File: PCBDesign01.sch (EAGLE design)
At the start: 94 parts, among them IC1 TESEO-LIV3R, J1 5051102491ACTUAL, U1 TPS71913-28DRVR, U2 FXOS8700CQR1, U3 CD40109BPWR, U4 MCP23017T-E/SO

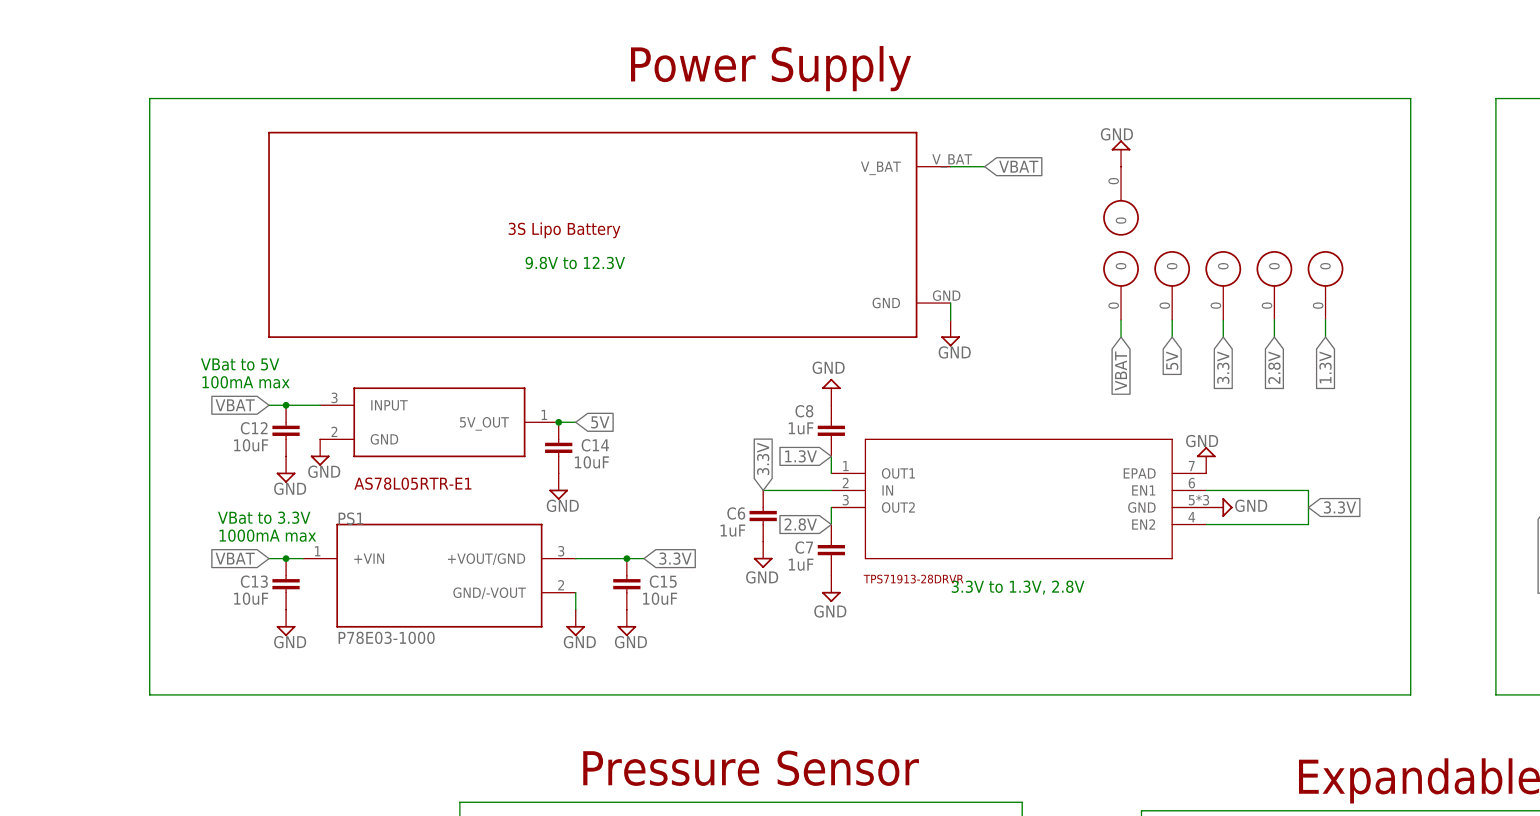
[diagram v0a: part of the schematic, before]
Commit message: final?
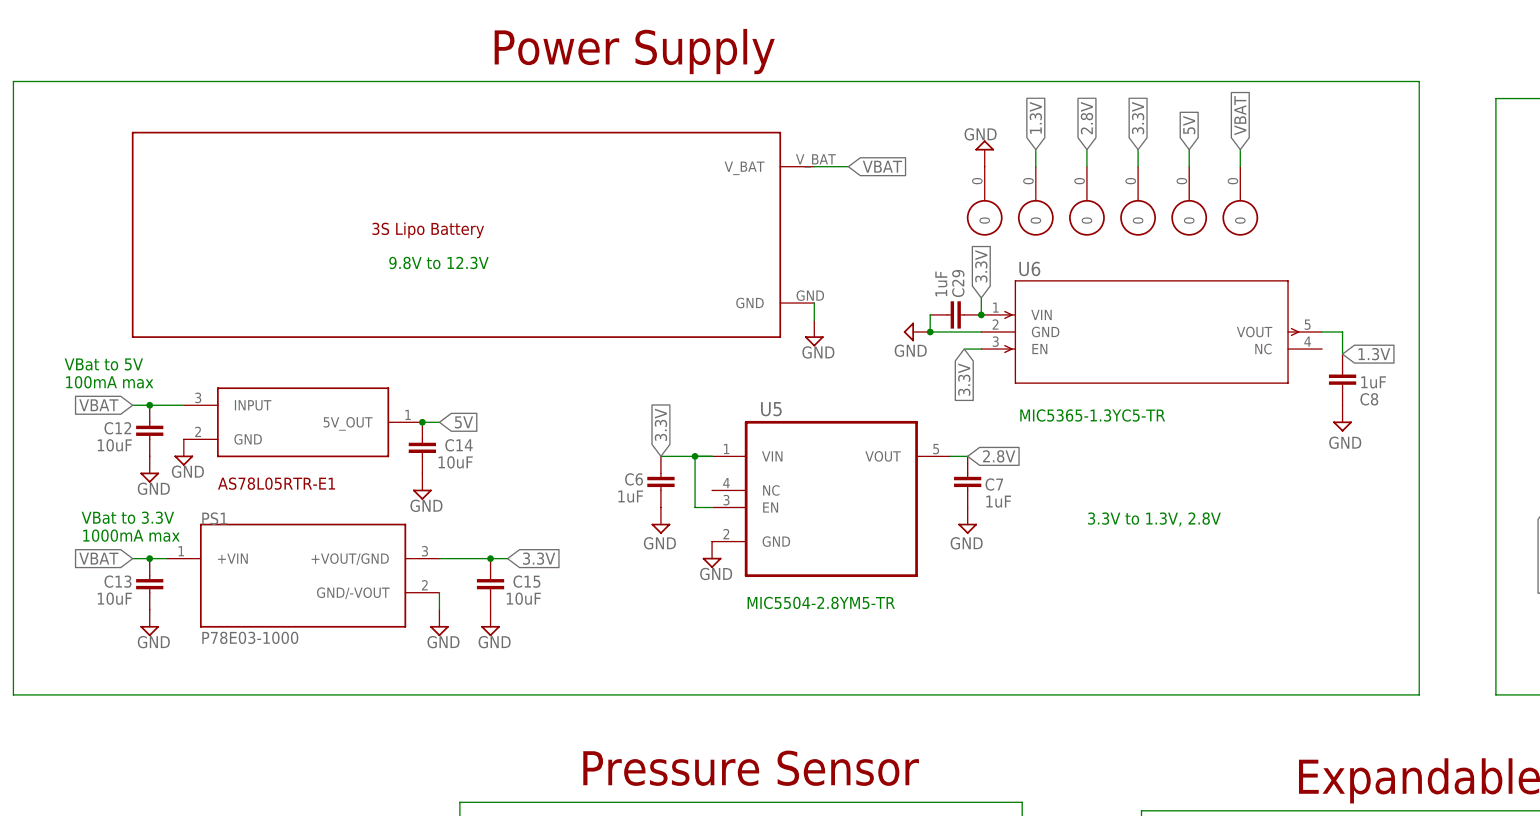
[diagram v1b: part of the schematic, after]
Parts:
- removed U1: TPS71913-28DRVR, TPS71913-28DRVR:TPS71913-28DRVR
- added C29: 1uF, Capacitor:C_CHIP-0805(2012-METRIC)
- added U5: MIC5504-2.8YM5-TR, MIC5504_2.8YM5:MIC5504-2.8YM5-TR
- added U6: MIC5365-1.3YC5-TRSC-70_C5_MCH-M, MIC5365_1.3YC5:MIC5365-1.3YC5-TRSC-70_C5_MCH-M
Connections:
- net 1.3V: now also U6.VOUT; no longer U1.OUT1
- net 2.8V: now also U5.VOUT; no longer U1.OUT2
- net 3.3V: now also C29.1, U5.EN, U5.VIN, U6.EN, U6.VIN; no longer U1.EN1, U1.EN2, U1.IN
- net GND: now also C29.2, U5.GND, U6.GND; no longer U1.EPAD, U1.GND
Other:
- note added: "MIC5365-1.3YC5-TR"
- note added: "MIC5504-2.8YM5-TR"
- moved on the sheet: C12, C13, C14, C15, C6, C7, C8, PS1
